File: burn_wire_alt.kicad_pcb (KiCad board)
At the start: 2 copper layers, 24.5 x 26 mm, 18 parts, among them J1 TestPoint_THTPad_1.0x1.0mm_Dr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, J2 TestPoint_THTPad_1.0x1.0mm_Dr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, U1 ADP2303ARDZ

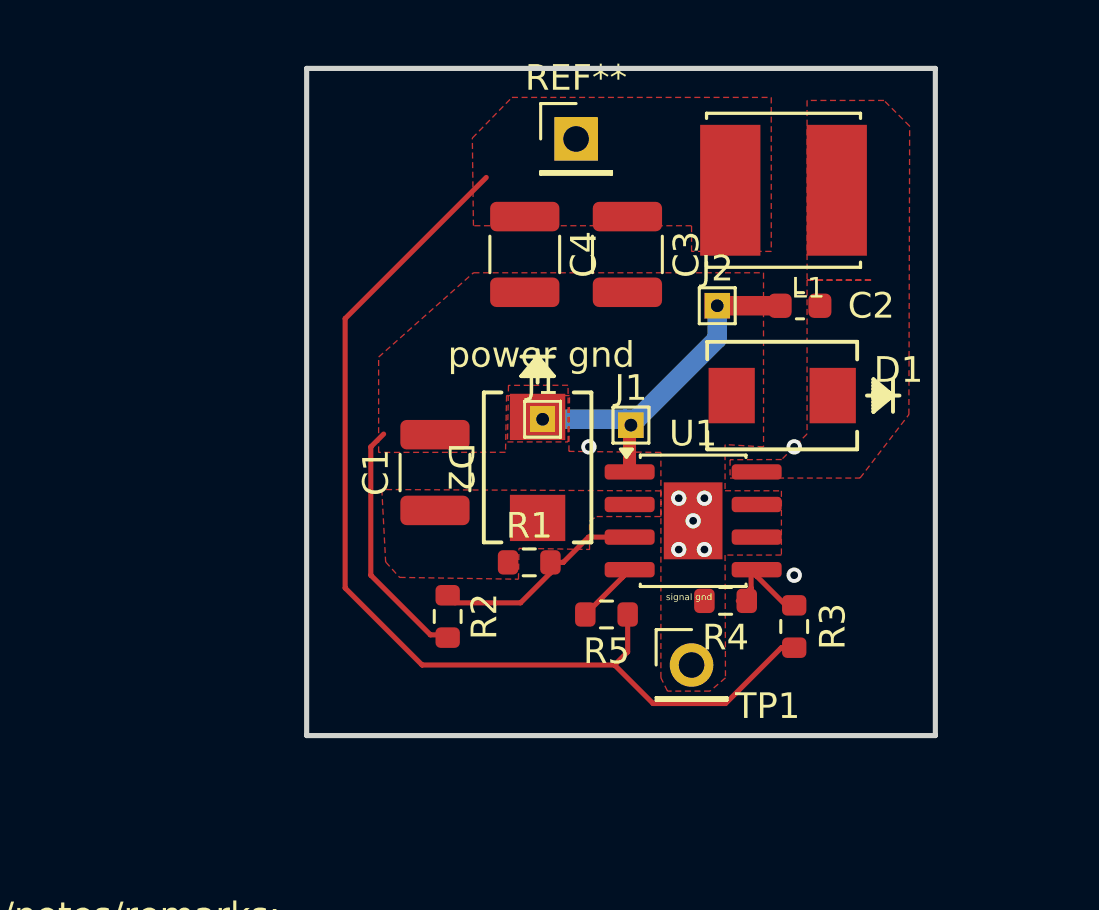
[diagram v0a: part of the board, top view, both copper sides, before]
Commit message: applied .gitignore
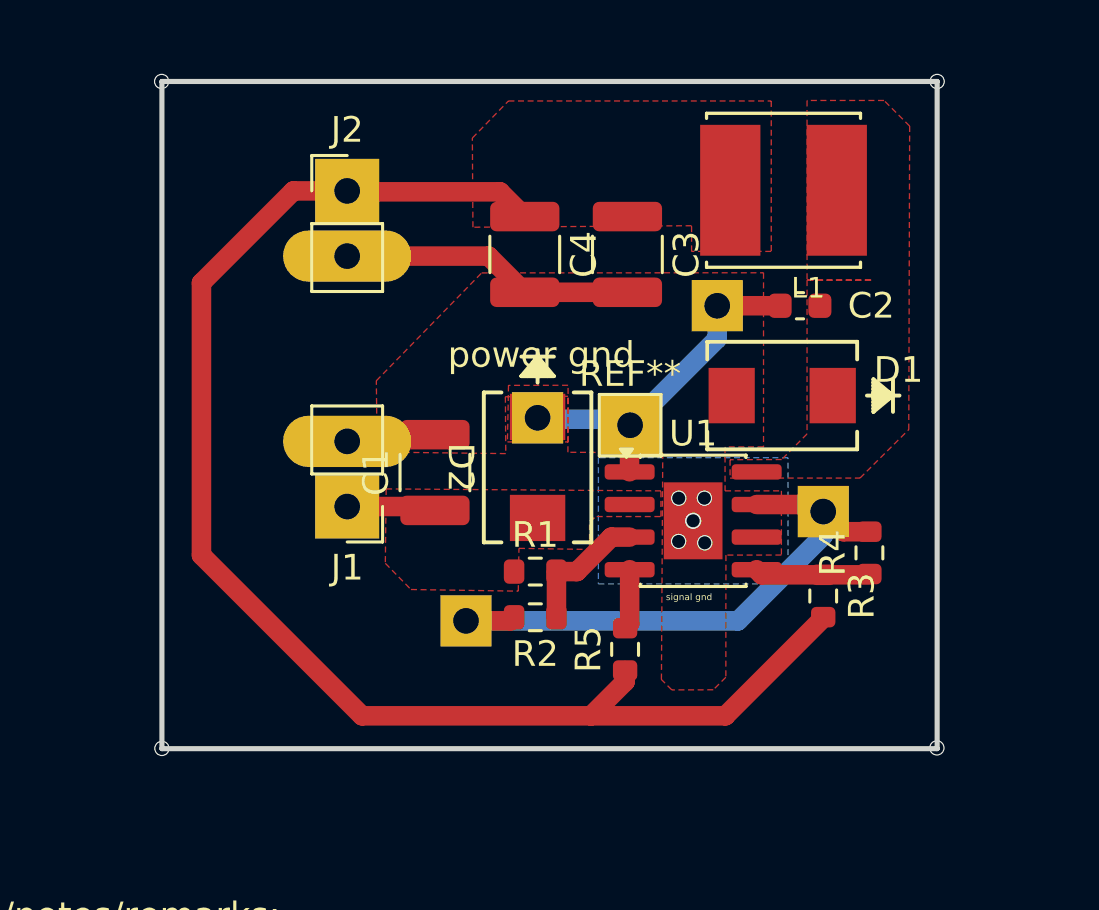
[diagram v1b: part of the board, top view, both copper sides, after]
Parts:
- removed the J1 at (164.7, 90.4)
- removed the J1 at (168.1, 90.7)
- removed the REF** at (166.0, 79.5)
- removed TP1: PinHeader_1x01_P2.54mm_Vertical, Connector_PinHeader_2.54mm:PinHeader_1x01_P2.54mm_Vertical
- added ?: , , F.Cu at (164.5, 90.4)
- added ?: , , F.Cu at (171.5, 86.0)
- added ?: , , F.Cu at (175.6, 94.0)
- added ?: , , F.Cu at (161.7, 98.3)
- added J1: Conn_01x02_Pin, Connector_PinHeader_2.54mm:PinHeader_1x02_P2.54mm_Vertical, F.Cu at (157.1, 93.8)
- added REF**: TestPoint_THTPad_2.0x2.0mm_Drill1.0mm, TestPoint:TestPoint_THTPad_2.0x2.0mm_Drill1.0mm, F.Cu at (168.1, 90.7)
- J2: value TestPoint_THTPad_1.0x1.0mm_Drill0.5mm -> Conn_01x02_Pin; footprint TestPoint:TestPoint_THTPad_1.0x1.0mm_Drill0.5mm -> Connector_PinHeader_2.54mm:PinHeader_1x02_P2.54mm_Vertical
- moved J2 15.1 mm to (157.1, 81.5)
- moved R4 5.91 mm to (177.4, 95.6), turned to 90 degrees
- moved R2 3.41 mm to (164.4, 98.1), turned to 180 degrees
- moved R3 1.64 mm to (175.6, 97.3)
- moved R5 1.54 mm to (167.9, 99.4), turned to 90 degrees
- moved R1 0.43 mm to (164.4, 96.4)
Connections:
- J2 pad 1: /BST -> /Vout
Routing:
- net GND: track 9.92 -> 38.1 mm, vias 6 -> 9
- net /Vout: track 40.7 -> 55.9 mm
- net /Vin: track 0.00 -> 3.48 mm
- net /EN: track 8.21 -> 5.19 mm
- net /FB: track 3.70 -> 4.49 mm, vias 1 -> 0
- net /SW: vias 1 -> 0
- added copper zone on B.Cu, net GND
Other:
- board size 24.5 x 26 mm -> 30.2 x 26 mm
